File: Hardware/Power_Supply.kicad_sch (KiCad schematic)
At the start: 63 parts, among them J1 ICSP, J2 Conn_01x01, J3 Conn_01x01, J4 Screw_Terminal_01x02, J6 Conn_01x04, J7 Conn_01x04, SW1 UP, SW2 DW, SW3 V_I_SEL, SW4 O_EN, U1 L78L08_SOT89, U2 ATmega328PB-AU, U3 TPS54531DDAR, U4 LM358, U5 INA138, U6 MCP4023-103ECH, Y1 16MHz

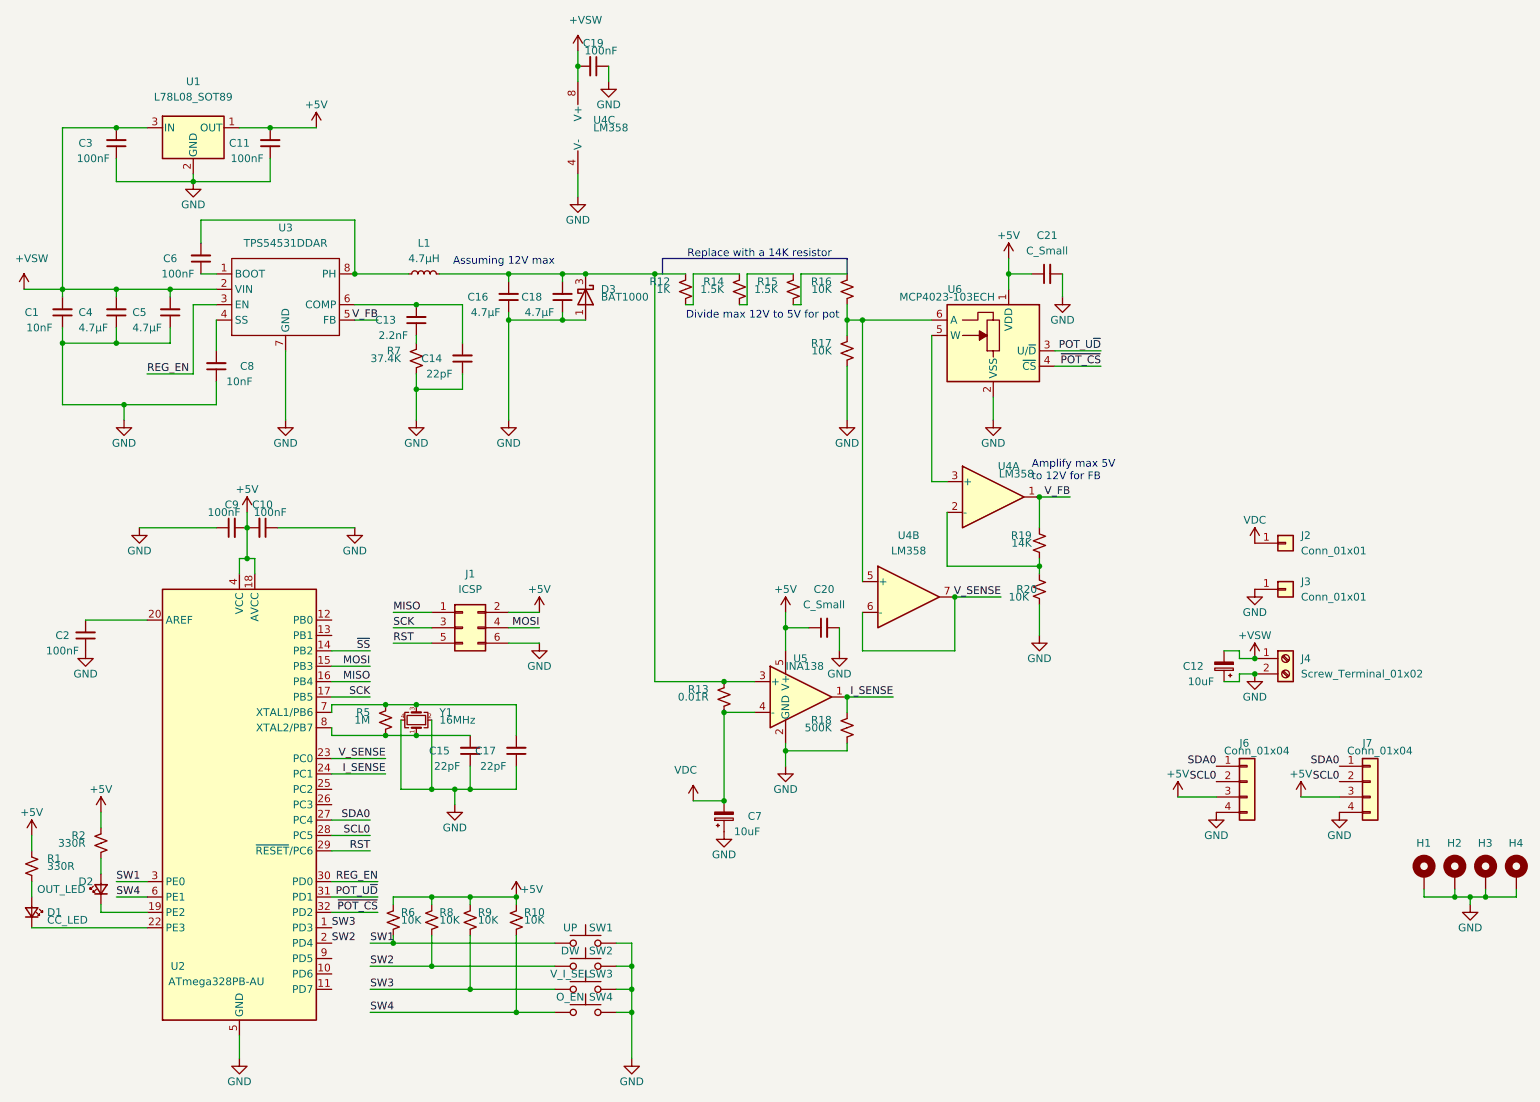
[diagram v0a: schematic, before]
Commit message: working on 3-d model
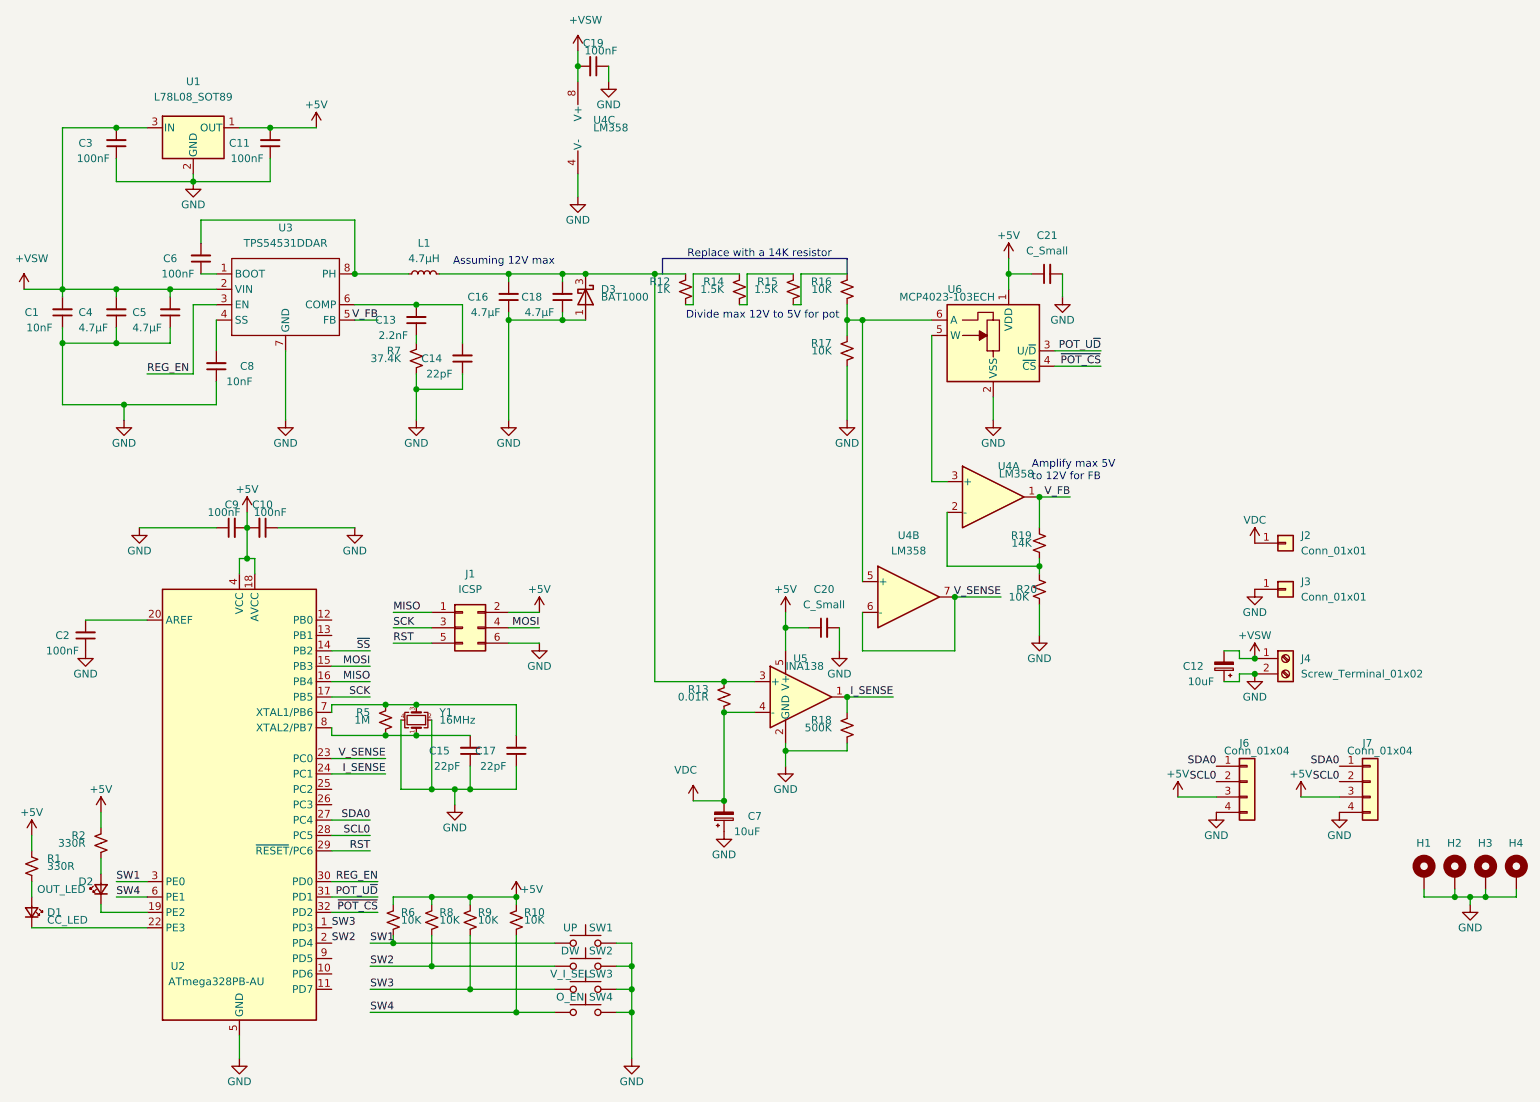
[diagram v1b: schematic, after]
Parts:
- U3: footprint Package_SO:SOIC-8-1EP_3.9x4.9mm_P1.27mm_EP2.514x3.2mm_ThermalVias -> Package_SO:SOIC-8-1EP_3.9x4.9mm_P1.27mm_EP2.514x3.2mm
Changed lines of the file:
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@@
-(kicad_sch (version 20200714) (host eeschema "(5.99.0-2441-g41b7c7c43)")
+(kicad_sch (version 20200714) (host eeschema "(5.99.0-2619-gb519867d9)")
   (page 1 1)
   (paper "A4")
-  (junction (at 22.86 58.42) (diameter 0) (color 0 0 0 0))
-  (junction (at 22.86 67.31) (diameter 0) (color 0 0 0 0))
-  (junction (at 31.75 31.75) (diameter 0) (color 0 0 0 0))
-  (junction (at 31.75 58.42) (diameter 0) (color 0 0 0 0))
-  (junction (at 31.75 67.31) (diameter 0) (color 0 0 0 0))
-  (junction (at 33.02 77.47) (diameter 0) (color 0 0 0 0))
-  (junction (at 40.64 58.42) (diameter 0) (color 0 0 0 0))
-  (junction (at 44.45 40.64) (diameter 0) (color 0 0 0 0))
-  (junction (at 53.34 97.79) (diameter 0) (color 0 0 0 0))
-  (junction (at 53.34 102.87) (diameter 0) (color 0 0 0 0))
-  (junction (at 57.15 31.75) (diameter 0) (color 0 0 0 0))
-  (junction (at 71.12 55.88) (diameter 0) (color 0 0 0 0))
-  (junction (at 76.2 127) (diameter 0) (color 0 0 0 0))
-  (junction (at 76.2 132.08) (diameter 0) (color 0 0 0 0))
-  (junction (at 77.47 166.37) (diameter 0) (color 0 0 0 0))
-  (junction (at 81.28 60.96) (diameter 0) (color 0 0 0 0))
-  (junction (at 81.28 74.93) (diameter 0) (color 0 0 0 0))
-  (junction (at 81.28 127) (diameter 0) (color 0 0 0 0))
-  (junction (at 81.28 132.08) (diameter 0) (color 0 0 0 0))
-  (junction (at 83.82 140.97) (diameter 0) (color 0 0 0 0))
-  (junction (at 83.82 158.75) (diameter 0) (color 0 0 0 0))
-  (junction (at 83.82 170.18) (diameter 0) (color 0 0 0 0))
-  (junction (at 87.63 140.97) (diameter 0) (color 0 0 0 0))
-  (junction (at 90.17 140.97) (diameter 0) (color 0 0 0 0))
-  (junction (at 90.17 158.75) (diameter 0) (color 0 0 0 0))
-  (junction (at 90.17 173.99) (diameter 0) (color 0 0 0 0))
-  (junction (at 96.52 55.88) (diameter 0) (color 0 0 0 0))
-  (junction (at 96.52 63.5) (diameter 0) (color 0 0 0 0))
-  (junction (at 97.79 158.75) (diameter 0) (color 0 0 0 0))
-  (junction (at 97.79 177.8) (diameter 0) (color 0 0 0 0))
-  (junction (at 105.41 55.88) (diameter 0) (color 0 0 0 0))
-  (junction (at 105.41 63.5) (diameter 0) (color 0 0 0 0))
-  (junction (at 107.95 21.59) (diameter 0) (color 0 0 0 0))
-  (junction (at 109.22 55.88) (diameter 0) (color 0 0 0 0))
-  (junction (at 116.84 170.18) (diameter 0) (color 0 0 0 0))
-  (junction (at 116.84 173.99) (diameter 0) (color 0 0 0 0))
-  (junction (at 116.84 177.8) (diameter 0) (color 0 0 0 0))
-  (junction (at 120.65 55.88) (diameter 0) (color 0 0 0 0))
-  (junction (at 132.08 123.19) (diameter 0) (color 0 0 0 0))
-  (junction (at 132.08 128.27) (diameter 0) (color 0 0 0 0))
-  (junction (at 132.08 142.875) (diameter 0) (color 0 0 0 0))
-  (junction (at 142.24 114.3) (diameter 0) (color 0 0 0 0))
-  (junction (at 142.24 134.62) (diameter 0) (color 0 0 0 0))
-  (junction (at 152.4 63.5) (diameter 0) (color 0 0 0 0))
-  (junction (at 152.4 125.73) (diameter 0) (color 0 0 0 0))
-  (junction (at 154.94 63.5) (diameter 0) (color 0 0 0 0))
-  (junction (at 170.18 109.22) (diameter 0) (color 0 0 0 0))
-  (junction (at 179.07 55.88) (diameter 0) (color 0 0 0 0))
-  (junction (at 184.15 92.71) (diameter 0) (color 0 0 0 0))
-  (junction (at 184.15 104.14) (diameter 0) (color 0 0 0 0))
-  (junction (at 219.71 119.38) (diameter 0) (color 0 0 0 0))
-  (junction (at 219.71 121.92) (diameter 0) (color 0 0 0 0))
-  (junction (at 252.73 158.75) (diameter 0) (color 0 0 0 0))
-  (junction (at 255.27 158.75) (diameter 0) (color 0 0 0 0))
-  (junction (at 257.81 158.75) (diameter 0) (color 0 0 0 0))
+  (junction (at 22.86 58.42) (diameter 1.016) (color 0 0 0 0))
+  (junction (at 22.86 67.31) (diameter 1.016) (color 0 0 0 0))
+  (junction (at 31.75 31.75) (diameter 1.016) (color 0 0 0 0))
+  (junction (at 31.75 58.42) (diameter 1.016) (color 0 0 0 0))
+  (junction (at 31.75 67.31) (diameter 1.016) (color 0 0 0 0))
+  (junction (at 33.02 77.47) (diameter 1.016) (color 0 0 0 0))
+  (junction (at 40.64 58.42) (diameter 1.016) (color 0 0 0 0))
+  (junction (at 44.45 40.64) (diameter 1.016) (color 0 0 0 0))
+  (junction (at 53.34 97.79) (diameter 1.016) (color 0 0 0 0))
+  (junction (at 53.34 102.87) (diameter 1.016) (color 0 0 0 0))
+  (junction (at 57.15 31.75) (diameter 1.016) (color 0 0 0 0))
+  (junction (at 71.12 55.88) (diameter 1.016) (color 0 0 0 0))
+  (junction (at 76.2 127) (diameter 1.016) (color 0 0 0 0))
+  (junction (at 76.2 132.08) (diameter 1.016) (color 0 0 0 0))
+  (junction (at 77.47 166.37) (diameter 1.016) (color 0 0 0 0))
+  (junction (at 81.28 60.96) (diameter 1.016) (color 0 0 0 0))
+  (junction (at 81.28 74.93) (diameter 1.016) (color 0 0 0 0))
+  (junction (at 81.28 127) (diameter 1.016) (color 0 0 0 0))
+  (junction (at 81.28 132.08) (diameter 1.016) (color 0 0 0 0))
+  (junction (at 83.82 140.97) (diameter 1.016) (color 0 0 0 0))
+  (junction (at 83.82 158.75) (diameter 1.016) (color 0 0 0 0))
+  (junction (at 83.82 170.18) (diameter 1.016) (color 0 0 0 0))
+  (junction (at 87.63 140.97) (diameter 1.016) (color 0 0 0 0))
+  (junction (at 90.17 140.97) (diameter 1.016) (color 0 0 0 0))
+  (junction (at 90.17 158.75) (diameter 1.016) (color 0 0 0 0))
+  (junction (at 90.17 173.99) (diameter 1.016) (color 0 0 0 0))
+  (junction (at 96.52 55.88) (diameter 1.016) (color 0 0 0 0))
+  (junction (at 96.52 63.5) (diameter 1.016) (color 0 0 0 0))
+  (junction (at 97.79 158.75) (diameter 1.016) (color 0 0 0 0))
+  (junction (at 97.79 177.8) (diameter 1.016) (color 0 0 0 0))
+  (junction (at 105.41 55.88) (diameter 1.016) (color 0 0 0 0))
+  (junction (at 105.41 63.5) (diameter 1.016) (color 0 0 0 0))
+  (junction (at 107.95 21.59) (diameter 1.016) (color 0 0 0 0))
+  (junction (at 109.22 55.88) (diameter 1.016) (color 0 0 0 0))
+  (junction (at 116.84 170.18) (diameter 1.016) (color 0 0 0 0))
+  (junction (at 116.84 173.99) (diameter 1.016) (color 0 0 0 0))
+  (junction (at 116.84 177.8) (diameter 1.016) (color 0 0 0 0))
+  (junction (at 120.65 55.88) (diameter 1.016) (color 0 0 0 0))
+  (junction (at 132.08 123.19) (diameter 1.016) (color 0 0 0 0))
+  (junction (at 132.08 128.27) (diameter 1.016) (color 0 0 0 0))
+  (junction (at 132.08 142.875) (diameter 1.016) (color 0 0 0 0))
+  (junction (at 142.24 114.3) (diameter 1.016) (color 0 0 0 0))
+  (junction (at 142.24 134.62) (diameter 1.016) (color 0 0 0 0))
+  (junction (at 152.4 63.5) (diameter 1.016) (color 0 0 0 0))
+  (junction (at 152.4 125.73) (diameter 1.016) (color 0 0 0 0))
+  (junction (at 154.94 63.5) (diameter 1.016) (color 0 0 0 0))
+  (junction (at 170.18 109.22) (diameter 1.016) (color 0 0 0 0))
+  (junction (at 179.07 55.88) (diameter 1.016) (color 0 0 0 0))
+  (junction (at 184.15 92.71) (diameter 1.016) (color 0 0 0 0))
+  (junction (at 184.15 104.14) (diameter 1.016) (color 0 0 0 0))
+  (junction (at 219.71 119.38) (diameter 1.016) (color 0 0 0 0))
+  (junction (at 219.71 121.92) (diameter 1.016) (color 0 0 0 0))
+  (junction (at 252.73 158.75) (diameter 1.016) (color 0 0 0 0))
+  (junction (at 255.27 158.75) (diameter 1.016) (color 0 0 0 0))
+  (junction (at 257.81 158.75) (diameter 1.016) (color 0 0 0 0))
   (wire (pts (xy 16.51 58.42) (xy 22.86 58.42))
     (stroke (width 0) (type solid) (color 0 0 0 0))
@@
     (property "Reference" "U3" (id 0) (at 59.69 48.26 0))
     (property "Value" "TPS54531DDAR" (id 1) (at 59.69 50.8 0))
-    (property "Footprint" "Package_SO:SOIC-8-1EP_3.9x4.9mm_P1.27mm_EP2.514x3.2mm_ThermalVias" (id 2) (at 67.31 68.58 0)
-      (effects (font (size 1.27 1.27)) hide)
-    )
+    (property "Footprint" "Package_SO:SOIC-8-1EP_3.9x4.9mm_P1.27mm_EP2.514x3.2mm" (id 2) (at 67.31 68.58 0)
+      (effects (font (size 1.27 1.27)) hide)
+    )
